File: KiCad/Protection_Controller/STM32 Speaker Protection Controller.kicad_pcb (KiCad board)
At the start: 2 copper layers, 121 x 182.2 mm, 62 parts, among them J1 AC1, J10 SPEAKER_OUT_R, J3 AC2, J5 AMP_OUT_L, J6 AMP_OUT_R, J8 SPEAKER_OUT_L, K1 G2RL-1A-E DC12, K2 G2RL-1A-E DC12, Q1 BC337, Q2 BC337, SW1 MUTE / ENABLE, SW2 FAULT RESET, T1 FS24-1500-C2, U1 LM7812, U2 NUCLEO-G031K8

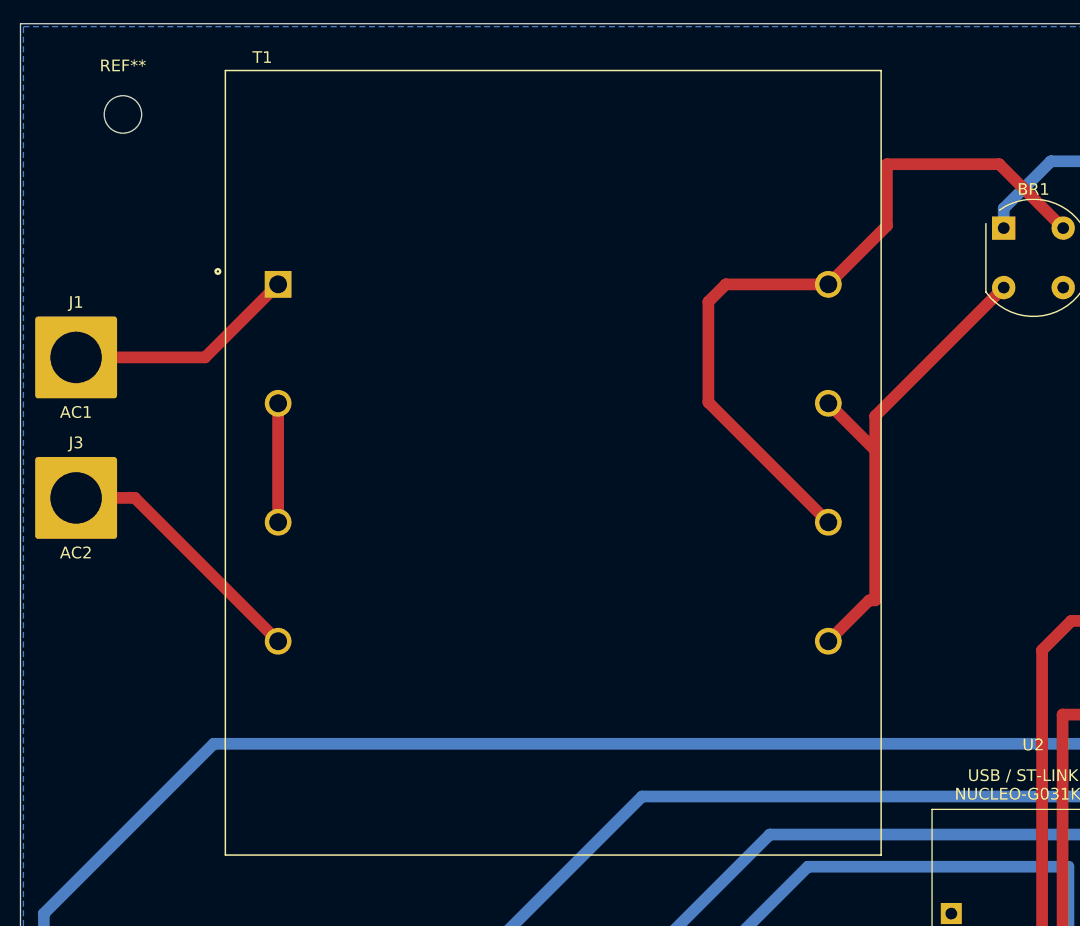
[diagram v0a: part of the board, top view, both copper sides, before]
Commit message: Add files via upload
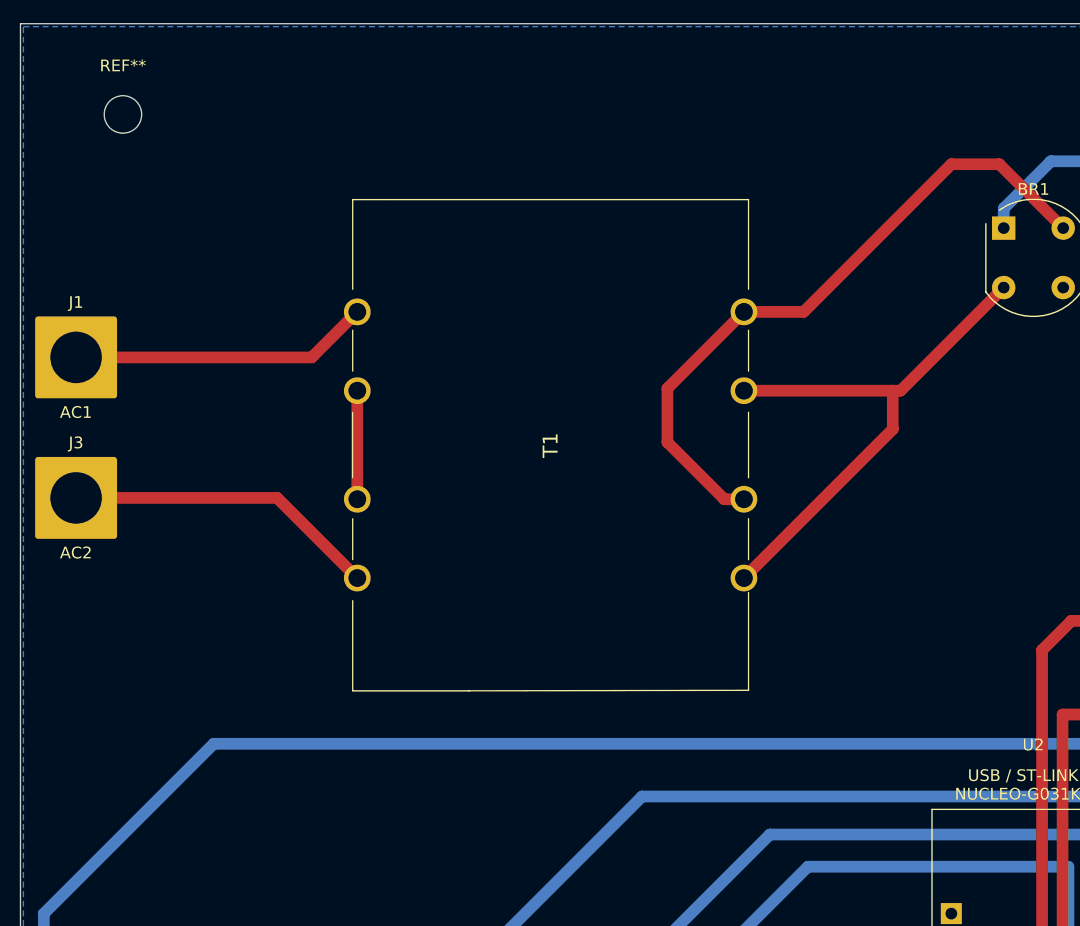
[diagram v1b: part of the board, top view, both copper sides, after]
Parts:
- T1: value FS24-1500-C2 -> FS24-250-C2; footprint FS24-1500-C2:TRANSFORMER_FS24-1500-C2 -> FS24-250-C2:FS24250C2
- moved T1 21.1 mm to (47.0, 39.4), turned to -90 degrees
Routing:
- net Net-(BR1-Pad4): track 63.6 -> 57.1 mm
- net Net-(J1-Pin_1): track 19.8 -> 25.6 mm
- net Net-(BR1-Pad2): track 42.4 -> 47.1 mm
- net Net-(J3-Pin_1): track 22.3 -> 26.9 mm
- net Net-(T1-Pad2): track 10.2 -> 9.27 mm
